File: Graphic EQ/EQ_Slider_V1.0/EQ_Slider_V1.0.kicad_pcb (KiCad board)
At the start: 2 copper layers, 95.3 x 63.5 mm, 27 parts

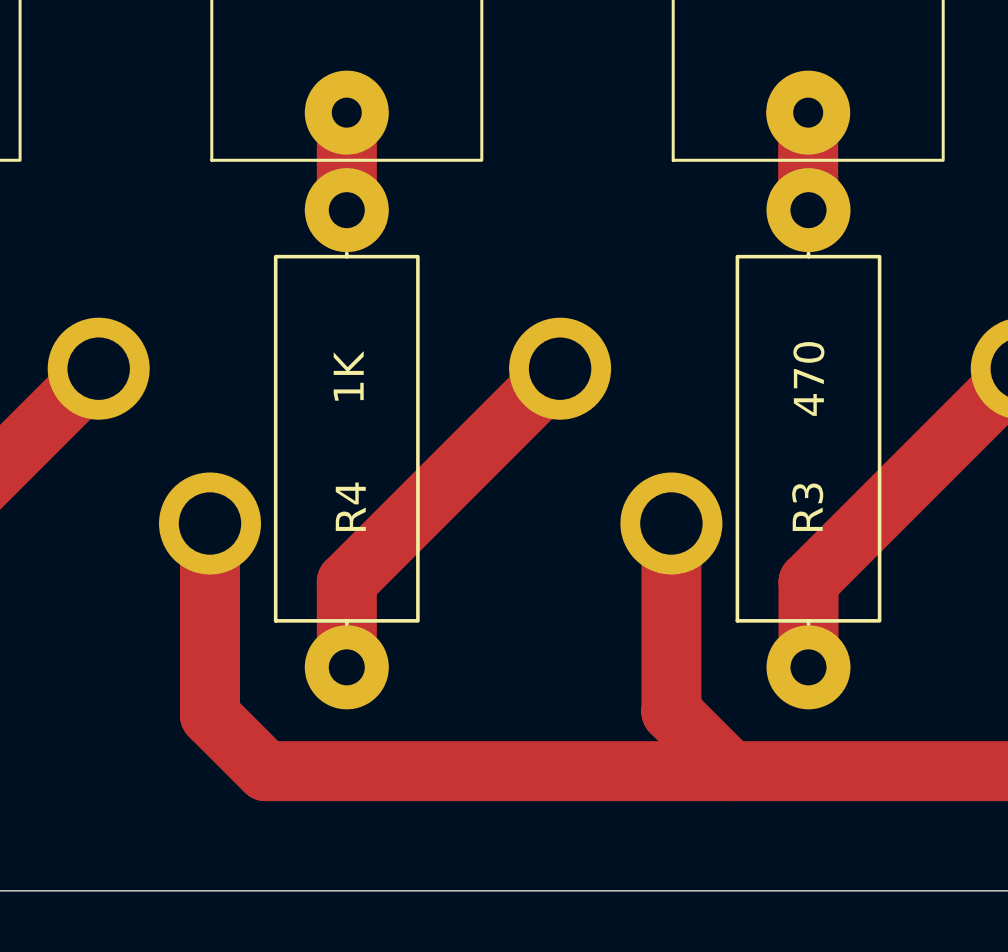
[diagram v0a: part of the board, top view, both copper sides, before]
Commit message: Preamp Progress, and Custom Footprint Library
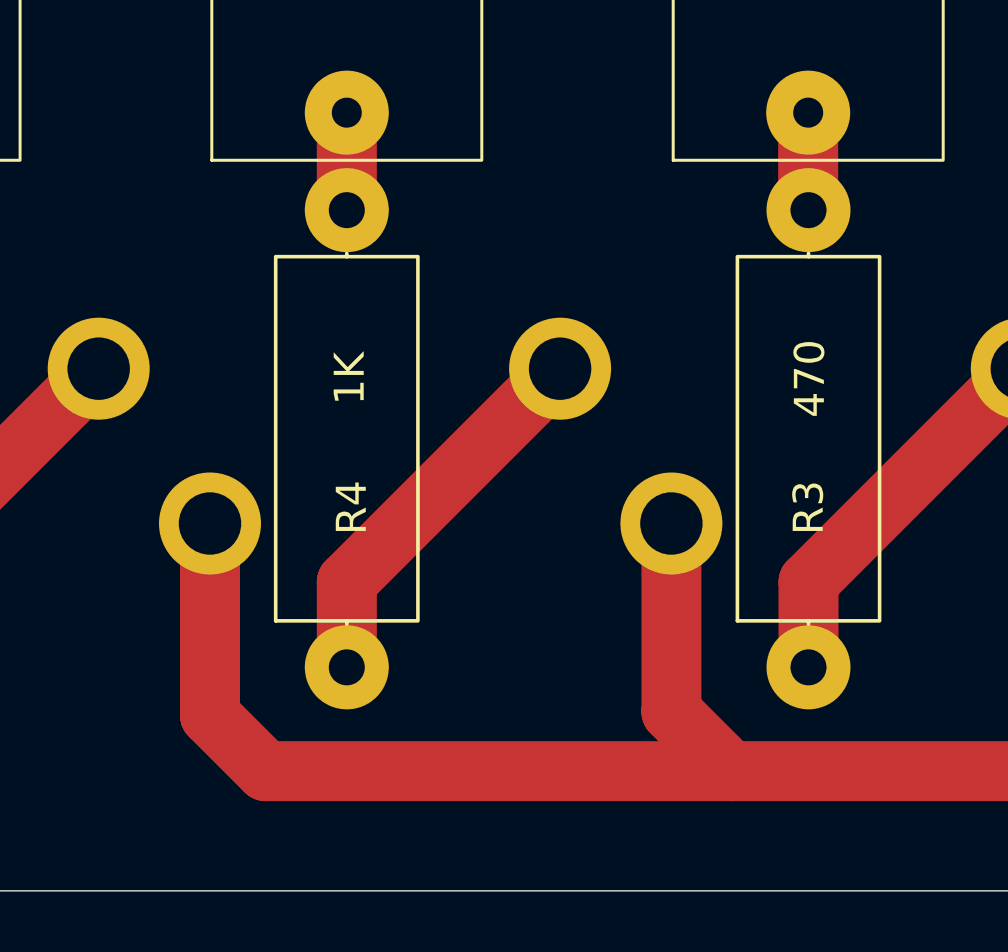
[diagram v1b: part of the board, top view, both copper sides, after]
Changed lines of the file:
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@@
-	)
-	(segment
-		(start 146.23 108.045)
-		(end 146.24 108.055)
-		(width 2)
-		(layer "F.Cu")
-		(net 10)
 	)
 	(segment
@@
 	)
 	(segment
-		(start 126.64 124.89)
-		(end 126.75 125)
-		(width 2)
-		(layer "F.Cu")
-		(net 15)
-	)
-	(segment
 		(start 157.41 124.66)
 		(end 159.5 126.75)
@@
 	)
 	(segment
-		(start 126.75 125)
+		(start 126.64 124.89)
 		(end 128.5 126.75)
 		(width 2)
